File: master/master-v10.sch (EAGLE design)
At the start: 44 parts

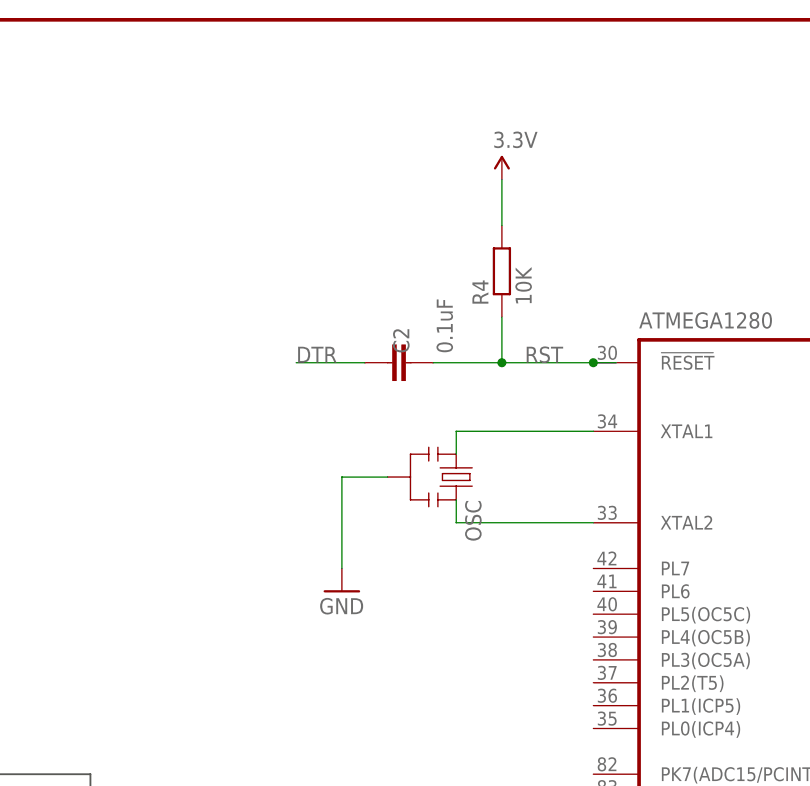
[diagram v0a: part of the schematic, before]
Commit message: add reset button
and rounded corners
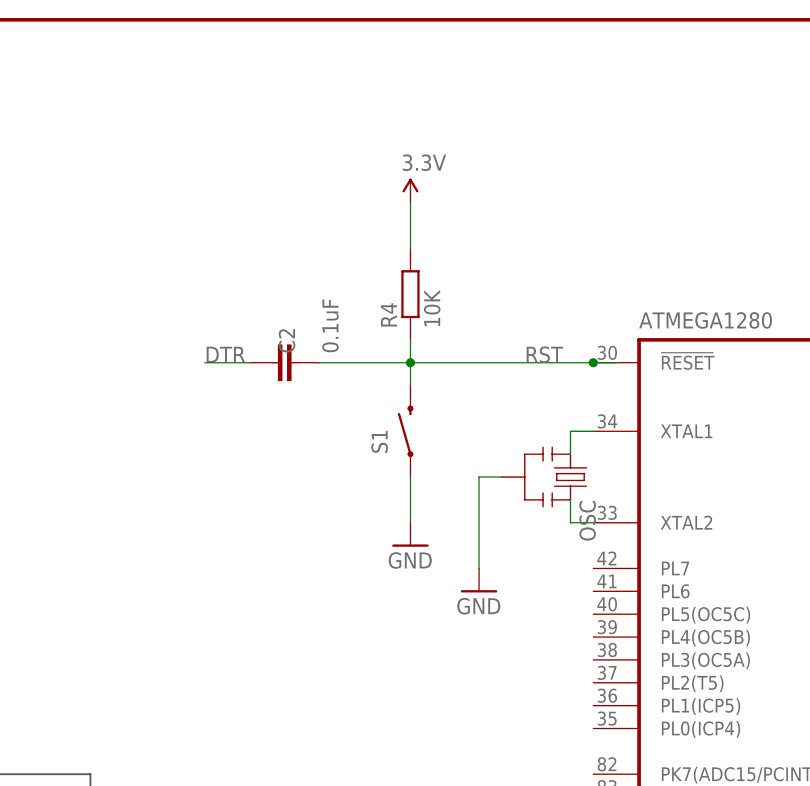
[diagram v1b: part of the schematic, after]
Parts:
- added S1: SWITCH-MOMENTARY-2-SMD-1101NE, SparkFun-Electromechanical:SWITCH-MOMENTARY-2-SMD-1101NE
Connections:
- net GND: now also S1.1
- net RST: now also S1.2
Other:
- moved on the sheet: C2, OSC, R4
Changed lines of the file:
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@@
 <part name="V_IN" library="holes" deviceset="MOUNT-PAD-ROUND" device="3.0"/>
 <part name="GND26" library="SparkFun" deviceset="GND" device=""/>
+<part name="S1" library="SparkFun-Electromechanical" deviceset="SWITCH-MOMENTARY-2" device="-SMD-1101NE"/>
+<part name="GND27" library="SparkFun" deviceset="GND" device=""/>
 </parts>
 <sheets>
@@
 <instance part="GND25" gate="1" x="71.12" y="238.76"/>
 <instance part="GND5" gate="1" x="172.72" y="66.04"/>
-<instance part="C2" gate="G$1" x="154.94" y="241.3" smashed="yes" rot="R270">
-<attribute name="NAME" x="154.813" y="242.316" size="1.778" layer="95" rot="R90"/>
-<attribute name="VALUE" x="159.639" y="242.316" size="1.778" layer="96" rot="R90"/>
+<instance part="C2" gate="G$1" x="142.24" y="241.3" smashed="yes" rot="R270">
+<attribute name="NAME" x="142.113" y="242.316" size="1.778" layer="95" rot="R90"/>
+<attribute name="VALUE" x="146.939" y="242.316" size="1.778" layer="96" rot="R90"/>
 </instance>
 <instance part="R1" gate="G$1" x="266.7" y="205.74" rot="R270"/>
@@
 <instance part="GND8" gate="1" x="7.62" y="38.1"/>
 <instance part="ATMEGA1280" gate="G$1" x="205.74" y="167.64"/>
-<instance part="R4" gate="G$1" x="165.1" y="251.46" rot="R90"/>
+<instance part="R4" gate="G$1" x="154.94" y="248.92" rot="R90"/>
 <instance part="DBG_L" gate="G$1" x="266.7" y="187.96"/>
 <instance part="PWR" gate="G$1" x="160.02" y="99.06"/>
@@
 <instance part="GND1" gate="1" x="302.26" y="243.84"/>
 <instance part="SUPPLY1" gate="G$1" x="76.2" y="256.54"/>
-<instance part="SUPPLY2" gate="G$1" x="165.1" y="261.62"/>
+<instance part="SUPPLY2" gate="G$1" x="154.94" y="259.08"/>
 <instance part="SUPPLY3" gate="G$1" x="7.62" y="81.28"/>
 <instance part="SUPPLY4" gate="G$1" x="154.94" y="127"/>
@@
 <instance part="FRAME1" gate="G$2" x="330.2" y="0"/>
 <instance part="3V3" gate="G$1" x="55.88" y="254"/>
-<instance part="GND18" gate="1" x="147.32" y="215.9"/>
+<instance part="GND18" gate="1" x="162.56" y="215.9"/>
 <instance part="R10" gate="G$1" x="292.1" y="154.94"/>
 <instance part="GND19" gate="1" x="304.8" y="129.54"/>
@@
 <instance part="GND16" gate="1" x="353.06" y="185.42" rot="R180"/>
 <instance part="SUPPLY10" gate="G$1" x="353.06" y="172.72" rot="R180"/>
-<instance part="OSC" gate="G$1" x="160.02" y="228.6" rot="R270"/>
+<instance part="OSC" gate="G$1" x="172.72" y="228.6" rot="R270"/>
 <instance part="JP2" gate="G$1" x="15.24" y="251.46"/>
 <instance part="GND17" gate="1" x="25.4" y="233.68"/>
@@
 <instance part="V_IN" gate="G$1" x="355.6" y="269.24"/>
 <instance part="GND26" gate="1" x="50.8" y="48.26"/>
+<instance part="S1" gate="G$1" x="154.94" y="233.68" smashed="yes" rot="R90">
+<attribute name="NAME" x="152.4" y="231.14" size="1.778" layer="95" rot="R90"/>
+</instance>
+<instance part="GND27" gate="1" x="154.94" y="220.98"/>
 </instances>
 <busses>
@@
 <segment>
 <pinref part="GND18" gate="1" pin="GND"/>
-<wire x1="152.4" y1="228.6" x2="147.32" y2="228.6" width="0.1524" layer="91"/>
-<wire x1="147.32" y1="228.6" x2="147.32" y2="218.44" width="0.1524" layer="91"/>
+<wire x1="165.1" y1="228.6" x2="162.56" y2="228.6" width="0.1524" layer="91"/>
+<wire x1="162.56" y1="228.6" x2="162.56" y2="218.44" width="0.1524" layer="91"/>
 <pinref part="OSC" gate="G$1" pin="2"/>
 </segment>
@@
 <pinref part="GND26" gate="1" pin="GND"/>
 </segment>
+<segment>
+<pinref part="GND27" gate="1" pin="GND"/>
+<pinref part="S1" gate="G$1" pin="1"/>
+<wire x1="154.94" y1="223.52" x2="154.94" y2="228.6" width="0.1524" layer="91"/>
+</segment>
 </net>
 <net name="SCK" class="0">
@@
 <net name="DTR" class="0">
 <segment>
-<wire x1="149.86" y1="241.3" x2="142.24" y2="241.3" width="0.1524" layer="91"/>
-<label x="142.24" y="241.3" size="1.778" layer="95"/>
+<wire x1="137.16" y1="241.3" x2="132.08" y2="241.3" width="0.1524" layer="91"/>
+<label x="132.08" y="241.3" size="1.778" layer="95"/>
 <pinref part="C2" gate="G$1" pin="2"/>
 </segment>
@@
 <segment>
 <wire x1="177.8" y1="241.3" x2="175.26" y2="241.3" width="0.1524" layer="91"/>
-<wire x1="175.26" y1="241.3" x2="165.1" y2="241.3" width="0.1524" layer="91"/>
-<wire x1="165.1" y1="241.3" x2="165.1" y2="246.38" width="0.1524" layer="91"/>
+<wire x1="175.26" y1="241.3" x2="154.94" y2="241.3" width="0.1524" layer="91"/>
+<wire x1="154.94" y1="241.3" x2="154.94" y2="243.84" width="0.1524" layer="91"/>
 <label x="167.64" y="241.3" size="1.778" layer="95"/>
 <pinref part="R4" gate="G$1" pin="1"/>
 <pinref part="C2" gate="G$1" pin="1"/>
-<wire x1="165.1" y1="241.3" x2="157.48" y2="241.3" width="0.1524" layer="91"/>
-<junction x="165.1" y="241.3"/>
+<wire x1="154.94" y1="241.3" x2="144.78" y2="241.3" width="0.1524" layer="91"/>
+<junction x="154.94" y="241.3"/>
 <pinref part="ATMEGA1280" gate="G$1" pin="!RESET!"/>
 <junction x="175.26" y="241.3"/>
+<pinref part="S1" gate="G$1" pin="2"/>
+<wire x1="154.94" y1="238.76" x2="154.94" y2="241.3" width="0.1524" layer="91"/>
 </segment>
 <segment>
@@
 <pinref part="R4" gate="G$1" pin="2"/>
 <pinref part="SUPPLY2" gate="G$1" pin="3.3V"/>
-<wire x1="165.1" y1="261.62" x2="165.1" y2="256.54" width="0.1524" layer="91"/>
+<wire x1="154.94" y1="259.08" x2="154.94" y2="254" width="0.1524" layer="91"/>
 </segment>
 <segment>
@@
 <net name="N$2" class="0">
 <segment>
-<wire x1="160.02" y1="233.68" x2="160.02" y2="231.14" width="0.1524" layer="91"/>
+<wire x1="172.72" y1="233.68" x2="172.72" y2="231.14" width="0.1524" layer="91"/>
 <pinref part="OSC" gate="G$1" pin="1"/>
 <pinref part="ATMEGA1280" gate="G$1" pin="XTAL1"/>
-<wire x1="160.02" y1="233.68" x2="175.26" y2="233.68" width="0.1524" layer="91"/>
+<wire x1="172.72" y1="233.68" x2="175.26" y2="233.68" width="0.1524" layer="91"/>
 </segment>
 </net>
@@
 <segment>
 <pinref part="ATMEGA1280" gate="G$1" pin="XTAL2"/>
-<wire x1="175.26" y1="223.52" x2="160.02" y2="223.52" width="0.1524" layer="91"/>
+<wire x1="175.26" y1="223.52" x2="172.72" y2="223.52" width="0.1524" layer="91"/>
 <pinref part="OSC" gate="G$1" pin="3"/>
-<wire x1="160.02" y1="223.52" x2="160.02" y2="226.06" width="0.1524" layer="91"/>
-</segment>
-</net>
+<wire x1="172.72" y1="223.52" x2="172.72" y2="226.06" width="0.1524" layer="91"/>
+</segment>
+</net>
